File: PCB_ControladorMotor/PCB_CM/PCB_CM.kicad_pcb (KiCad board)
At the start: 2 copper layers, 104.5 x 67.2 mm, 25 parts, among them J1 Conn_01x02_Socket, J2 Conn_01x02_Socket, J3 Conn_01x02_Socket, J4 Conn_01x02_Socket, Q1 IRF540N, U1 LM324A, U2 ATtiny85V-10P

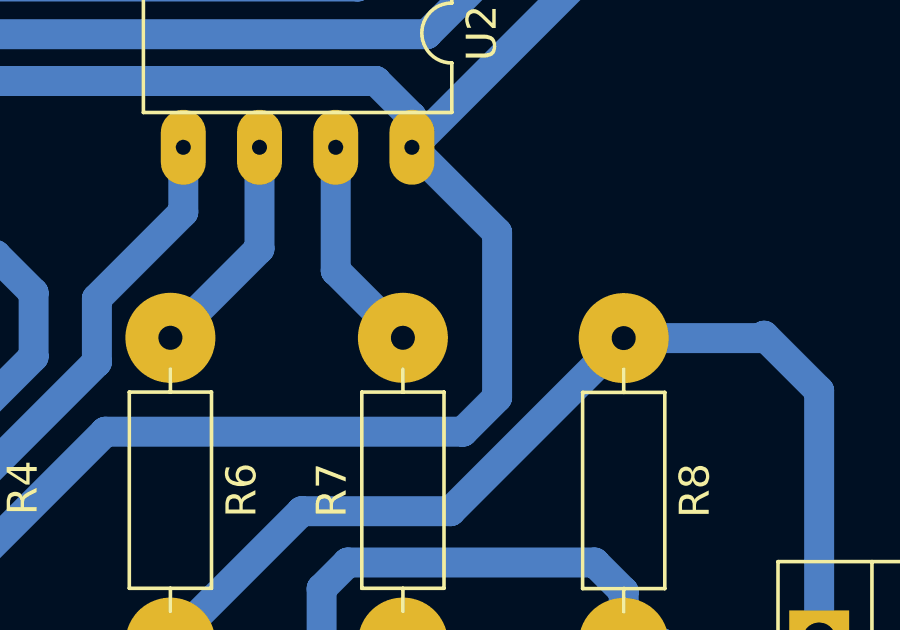
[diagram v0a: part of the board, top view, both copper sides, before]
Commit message: Add files via upload
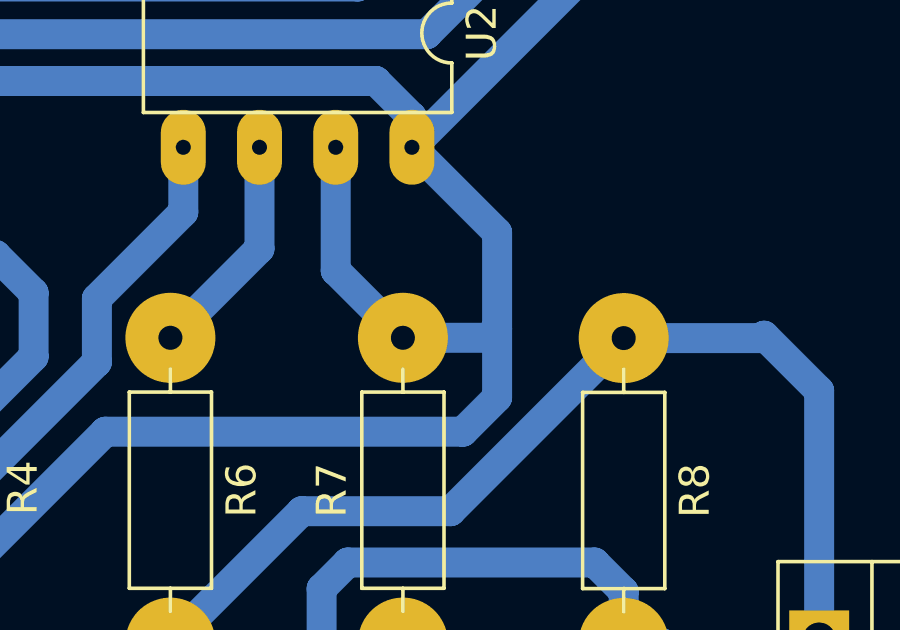
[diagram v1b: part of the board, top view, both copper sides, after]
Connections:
- R7 pad 2: Net-(U2-PB2) -> Net-(J3-Pin_2)
- U2 pad 7: Net-(U2-PB2) -> Net-(J3-Pin_2)
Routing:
- net Net-(J3-Pin_2): track 102.0 -> 112.5 mm
- net Net-(U2-PB2): track 7.28 -> 0.00 mm
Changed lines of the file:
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@@
 	(net 13 "Net-(U2-AREF{slash}PB0)")
 	(net 14 "Net-(U2-PB1)")
-	(net 15 "Net-(U2-PB2)")
-	(net 16 "unconnected-(U2-XTAL2{slash}PB4-Pad3)")
-	(net 17 "Net-(U2-XTAL1{slash}PB3)")
+	(net 15 "unconnected-(U2-XTAL2{slash}PB4-Pad3)")
+	(net 16 "Net-(U2-XTAL1{slash}PB3)")
 	(footprint "MountingHole:MountingHole_2.2mm_M2_DIN965_Pad"
 		(layer "F.Cu")
@@
 			(layers "*.Cu" "*.Mask")
 			(remove_unused_layers no)
-			(net 15 "Net-(U2-PB2)")
+			(net 9 "Net-(J3-Pin_2)")
 			(pintype "passive")
 		)
@@
 			(layers "*.Cu" "*.Mask")
 			(remove_unused_layers no)
-			(net 17 "Net-(U2-XTAL1{slash}PB3)")
+			(net 16 "Net-(U2-XTAL1{slash}PB3)")
 			(pintype "passive")
 		)
@@
 			(layers "*.Cu" "*.Mask")
 			(remove_unused_layers no)
-			(net 17 "Net-(U2-XTAL1{slash}PB3)")
+			(net 16 "Net-(U2-XTAL1{slash}PB3)")
 			(pinfunction "XTAL1/PB3")
 			(pintype "bidirectional")
@@
 			(layers "*.Cu" "*.Mask")
 			(remove_unused_layers no)
-			(net 16 "unconnected-(U2-XTAL2{slash}PB4-Pad3)")
+			(net 15 "unconnected-(U2-XTAL2{slash}PB4-Pad3)")
 			(pinfunction "XTAL2/PB4")
 			(pintype "bidirectional")
@@
 			(layers "*.Cu" "*.Mask")
 			(remove_unused_layers no)
-			(net 15 "Net-(U2-PB2)")
+			(net 9 "Net-(J3-Pin_2)")
 			(pinfunction "PB2")
 			(pintype "bidirectional")
@@
 			(layers "*.Cu" "*.Mask")
 			(remove_unused_layers no)
-			(net 17 "Net-(U2-XTAL1{slash}PB3)")
+			(net 16 "Net-(U2-XTAL1{slash}PB3)")
 			(pintype "passive")
 		)
@@
 	)
 	(segment
+		(start 122.26 80.32)
+		(end 122.26 84.43)
+		(width 1)
+		(layer "B.Cu")
+		(net 9)
+	)
+	(segment
 		(start 127.64 88.66)
-		(end 127.64 83.16)
+		(end 127.64 86.36)
 		(width 1)
 		(layer "B.Cu")
@@
 	)
 	(segment
+		(start 127.33 86.67)
+		(end 127.64 86.36)
+		(width 1)
+		(layer "B.Cu")
+		(net 9)
+	)
+	(segment
 		(start 124.8 80.32)
 		(end 124.8 79.31)
@@
 	)
 	(segment
+		(start 124.5 86.67)
+		(end 127.33 86.67)
+		(width 1)
+		(layer "B.Cu")
+		(net 9)
+	)
+	(segment
 		(start 126.5 89.8)
 		(end 127.64 88.66)
@@
 	)
 	(segment
+		(start 127.64 86.36)
+		(end 127.64 83.16)
+		(width 1)
+		(layer "B.Cu")
+		(net 9)
+	)
+	(segment
+		(start 122.26 84.43)
+		(end 124.5 86.67)
+		(width 1)
+		(layer "B.Cu")
+		(net 9)
+	)
+	(segment
 		(start 132.85 72.27)
 		(end 124.8 80.32)
@@
 	)
 	(segment
-		(start 122.26 80.32)
-		(end 122.26 84.43)
-		(width 1)
-		(layer "B.Cu")
-		(net 15)
-	)
-	(segment
-		(start 122.26 84.43)
-		(end 124.5 86.67)
-		(width 1)
-		(layer "B.Cu")
-		(net 15)
-	)
-	(segment
 		(start 102.85 66.54)
 		(end 103 66.69)
 		(width 1)
 		(layer "B.Cu")
-		(net 17)
+		(net 16)
 	)
 	(segment
@@
 		(width 1)
 		(layer "B.Cu")
-		(net 17)
+		(net 16)
 	)
 	(segment
@@
 		(width 1)
 		(layer "B.Cu")
-		(net 17)
+		(net 16)
 	)
 	(segment
@@
 		(width 1)
 		(layer "B.Cu")
-		(net 17)
+		(net 16)
 	)
 	(segment
@@
 		(width 1)
 		(layer "B.Cu")
-		(net 17)
+		(net 16)
 	)
 	(segment
@@
 		(width 1)
 		(layer "B.Cu")
-		(net 17)
+		(net 16)
 	)
 )
